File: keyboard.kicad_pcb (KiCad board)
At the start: 2 copper layers, 116.7 x 27.8 mm, 24 parts, among them SW1 SW_Push, U1 ATmega32U4-A, Y1 16MHz

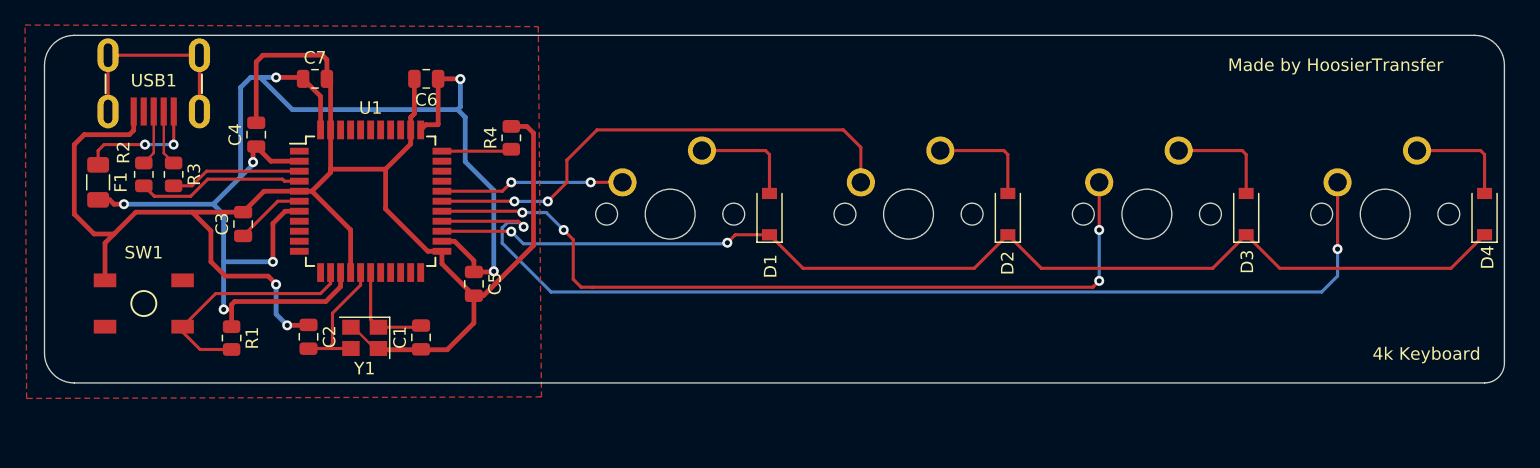
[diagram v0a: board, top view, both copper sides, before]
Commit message: f
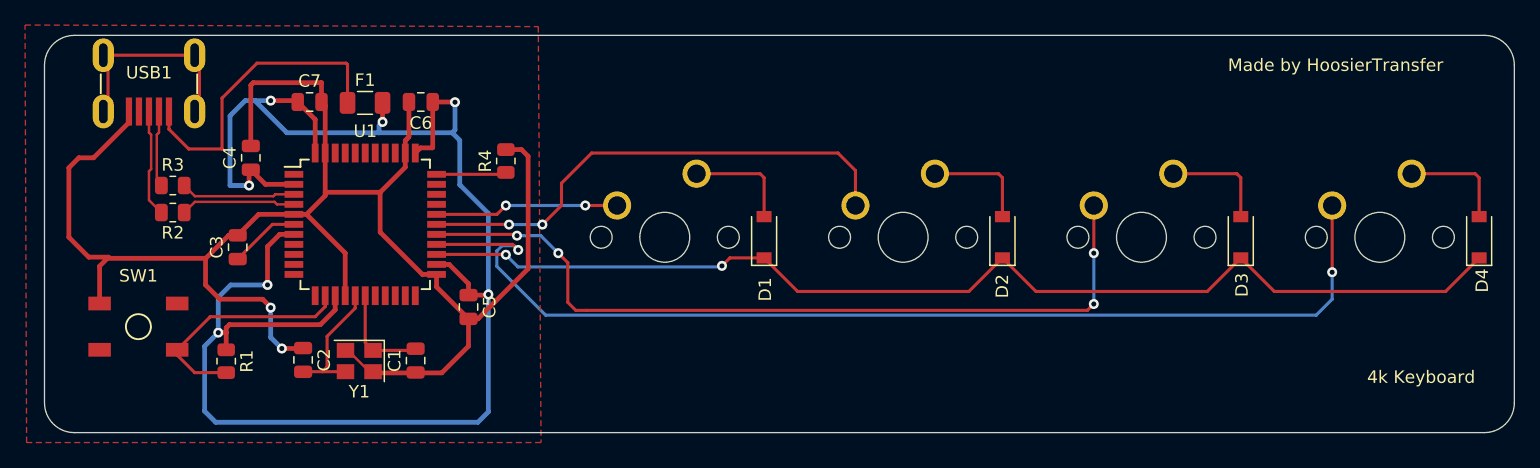
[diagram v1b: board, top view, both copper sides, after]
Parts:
- D1, D2, D4: value SOD-123 -> 1N4148W-TP
- moved F1 22.3 mm to (64.5, 80.0), turned to 0 degrees
- moved R2 3.83 mm to (49.1, 88.8), turned to 0 degrees
- moved C4 1.90 mm to (55.4, 84.4)
- moved R1 1.90 mm to (53.4, 100.7)
- moved Y1 1.90 mm to (64.1, 100.6)
- moved C3 1.90 mm to (54.3, 91.5)
- moved D4 1.90 mm to (153.6, 90.8)
- moved MX4 1.90 mm to (145.6, 90.8)
- moved C1 1.90 mm to (68.6, 100.6)
- moved C5 1.90 mm to (72.8, 96.3)
- moved C6 1.90 mm to (69.0, 79.9)
- moved C7 1.90 mm to (60.1, 79.9)
- moved D1 1.90 mm to (96.4, 90.8)
- moved D2 1.90 mm to (115.5, 90.8)
- moved MX1 1.90 mm to (88.5, 90.8)
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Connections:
- net Net-(R2-Pad2) renamed D0+
- net Net-(R3-Pad2) renamed D0-
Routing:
- net +5V: track 113.8 -> 136.8 mm
- net VCC: track 10.0 -> 24.7 mm, vias 2 -> 0
- net D0+: track 13.4 -> 9.20 mm
- net D+: track 4.44 -> 8.63 mm
- net GND: track 141.1 -> 138.9 mm
- net D-: track 4.44 -> 6.14 mm
- net D0-: track 10.5 -> 9.18 mm
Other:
- board size 116.7 x 27.8 mm -> 117.5 x 31.8 mm
